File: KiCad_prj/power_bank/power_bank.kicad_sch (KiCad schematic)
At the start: 2 parts, among them U2 TPS54560BDDA, U4 TPS54560BDDA

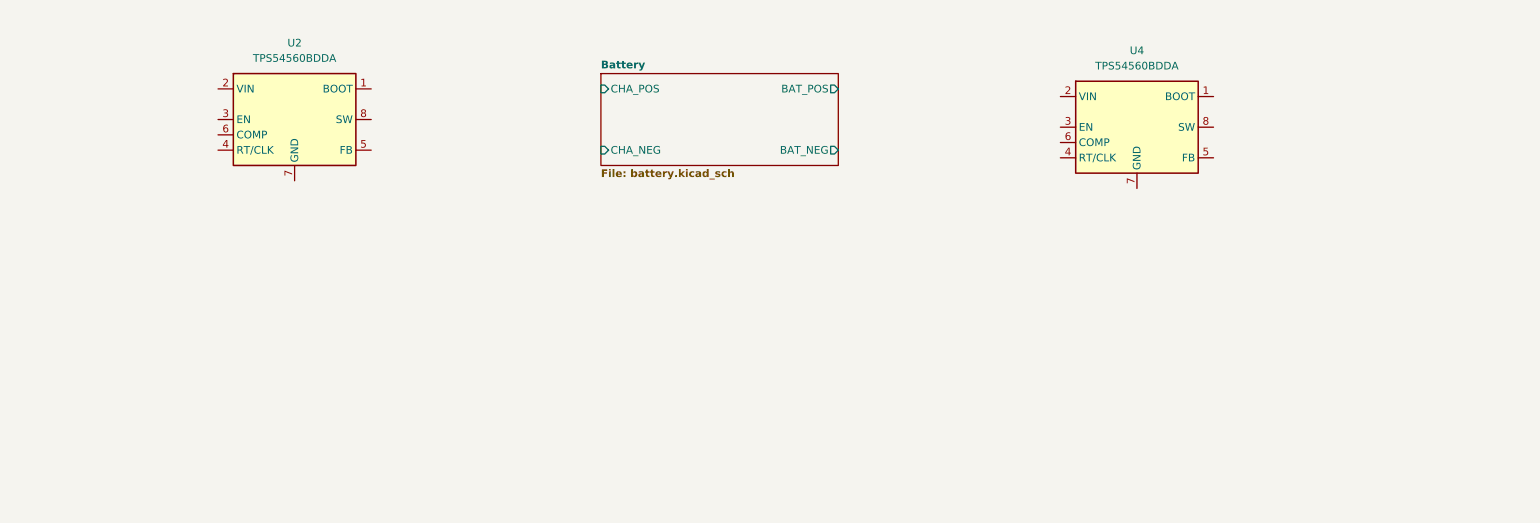
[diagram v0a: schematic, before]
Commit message: power_bank: dokonceny navrh schema
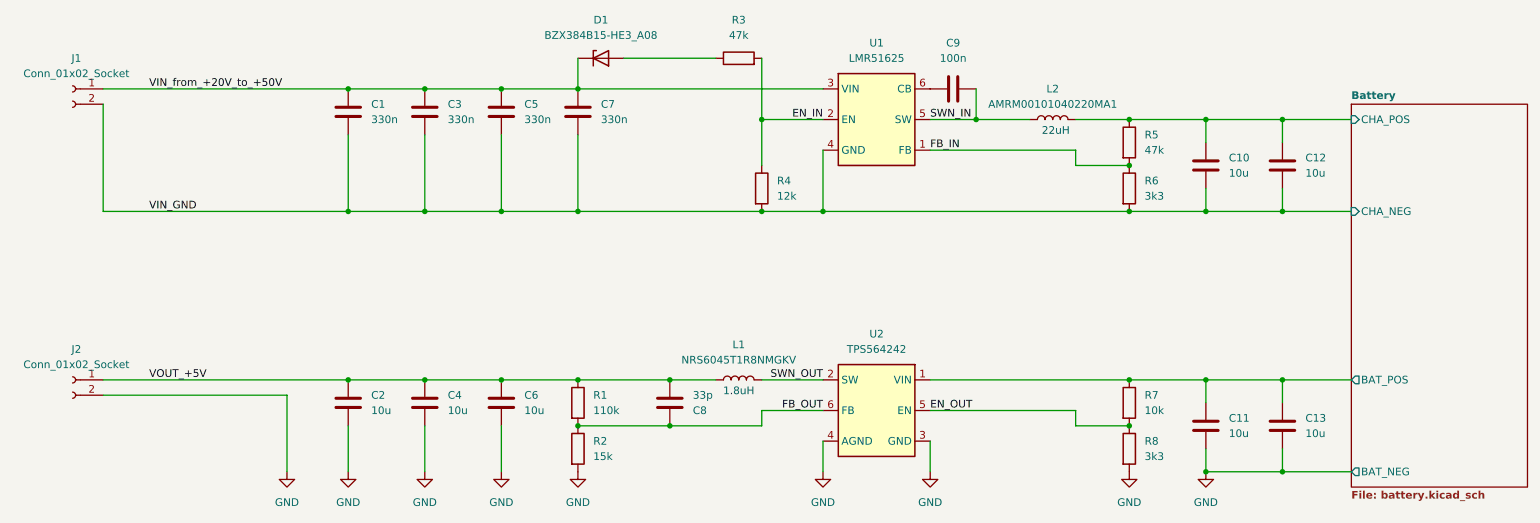
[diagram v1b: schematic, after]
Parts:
- removed U2, U4: TPS54560BDDA, Package_SO:Texas_R-PDSO-G8_EP2.95x4.9mm_Mask2.4x3.1mm_ThermalVias, symbol Regulator_Switching:TPS54560BDDA
- added C1, C3, C5, C7: 330n, symbol Device:C
- added C10, C11, C12, C13, C2, C4, C6: 10u, symbol Device:C
- added C8: 33p, symbol Device:C
- added C9: 100n, symbol Device:C
- added D1: BZX384B15-HE3_A08, Diode_SMD:D_SOD-323F, symbol Device:D_Zener
- added J1, J2: Conn_01x02_Socket, symbol Connector:Conn_01x02_Socket
- added L1: NRS6045T1R8NMGKV, symbol Device:L
- added L2: AMRM00101040220MA1, Inductor_SMD:L_10.4x10.4_H4.8, symbol Device:L
- added R1: 110k, Resistor_SMD:R_0805_2012Metric, symbol Device:R
- added R2: 15k, Resistor_SMD:R_0805_2012Metric, symbol Device:R
- added R3, R5: 47k, Resistor_SMD:R_0805_2012Metric, symbol Device:R
- added R4: 12k, Resistor_SMD:R_0805_2012Metric, symbol Device:R
- added R6, R8: 3k3, Resistor_SMD:R_0805_2012Metric, symbol Device:R
- added R7: 10k, Resistor_SMD:R_0805_2012Metric, symbol Device:R
- added U1: LMR51625, Package_TO_SOT_SMD:SOT-23-6, symbol switching_converters:LMR516x5
- added U2: TPS564242, Package_TO_SOT_SMD:SOT-563, symbol switching_converters:TPS564242
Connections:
- net Battery/BAT_POS: now also C11.1, C13.1, R7.1, U2.1 (VIN)
- net Battery/CHA_POS: now also C10.1, C12.1, L2.2, R5.1
- new net: C9.1, U1.6 (CB)
- new net: D1.2 (A), R3.1
- new net EN_IN: R3.2, R4.1, U1.2 (EN)
- new net EN_OUT: R7.2, R8.1, U2.5 (EN)
- new net FB_IN: R5.2, R6.1, U1.1 (FB)
- new net FB_OUT: C8.2, R1.2, R2.1, U2.6 (FB)
- new net GND: C11.2, C13.2, C2.2, C4.2, C6.2, J2.2 (Pin_2), R2.2, R8.2, U2.3 (GND), U2.4 (AGND)
- new net SWN_IN: C9.2, L2.1, U1.5 (SW)
- new net SWN_OUT: L1.2, U2.2 (SW)
- new net VIN_GND: C1.2, C10.2, C12.2, C3.2, C5.2, C7.2, J1.2 (Pin_2), R4.2, R6.2, U1.4 (GND)
- new net VIN_from_+20V_to_+50V: C1.1, C3.1, C5.1, C7.1, D1.1 (K), J1.1 (Pin_1), U1.3 (VIN)
- new net VOUT_+5V: C2.1, C4.1, C6.1, C8.1, J2.1 (Pin_1), L1.1, R1.1
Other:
- note added: "1.8uH"
- note added: "22uH"
- title: (none) -> ${TITLE}
